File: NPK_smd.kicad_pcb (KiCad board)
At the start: 2 copper layers, 64.2 x 85.9 mm, 59 parts, among them J1 DHT, J2 Screw_Terminal_01x04, J3 USB_C_Receptacle_USB2.0_16P, Q3 SS8050, Q4 SS8050, SW1 SW_Push, SW2 SW_Push, SW3 SW_SPST, U1 AMS1117-3.3, U2 MAX485ESA_T, U3 LM2596S-ADJ, U4 ESP32-WROOM-32, U6 USBLC6-2SC6, U7 CH340C

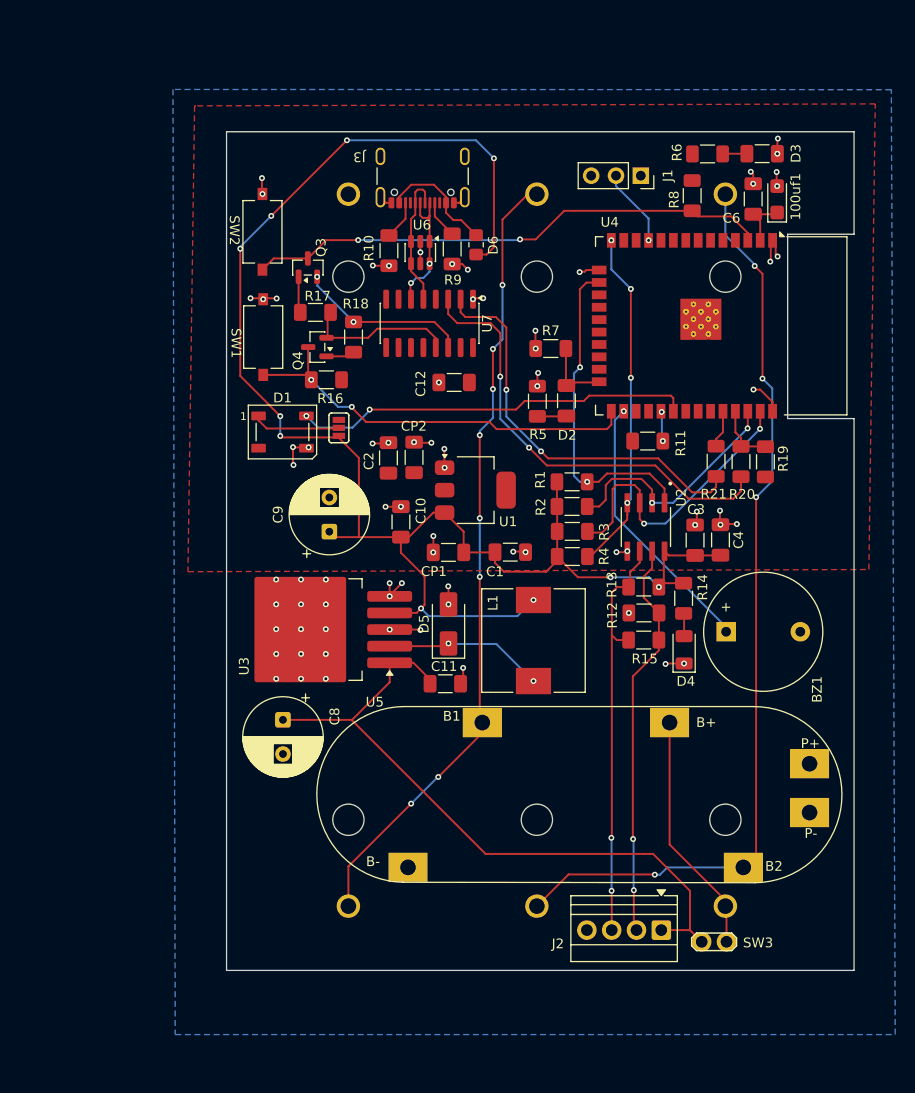
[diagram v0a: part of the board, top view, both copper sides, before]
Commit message: size minimizations and updations
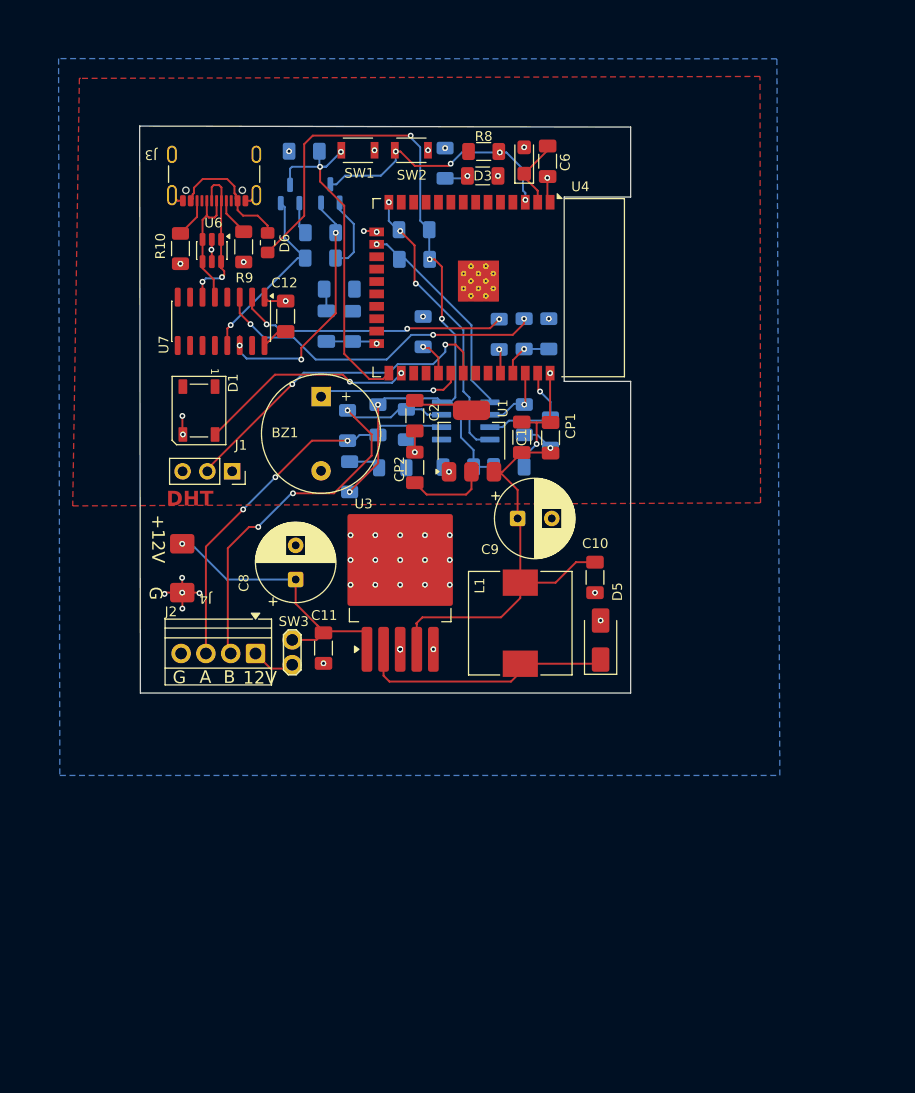
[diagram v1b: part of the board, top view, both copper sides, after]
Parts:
- removed BT2: BK-18650-PC6, 18650-3cell holder:BAT_BK-18650-PC6
- removed JP1: Jumper_3_Open, PCM_SparkFun-Jumper:Jumper_3_NO
- removed U5: ~, custom:BMS-10A-3S
- added G***: LOGO, LOGO, B.Cu at (130.1, 87.3)
- added G***: LOGO, LOGO, B.Cu at (106.3, 60.2)
- added J4: Conn_01x02_Pin, custom:solder-pad, F.Cu at (104.9, 88.3)
- added REF**: ESD-Logo_6.6x6mm_SilkScreen, Symbol:ESD-Logo_6.6x6mm_SilkScreen, B.Cu at (106.0, 69.3)
- C3, C4, D2, D4, Q3, Q4, R1, R11, R12, R13, R14, R15, R16, R17, R18, R19, R2, R20, R21, R3, R4, R5, R6, R7, U2: moved to B.Cu
- SW1, SW2: footprint Button_Switch_SMD:SW_Tactile_SPST_NO_Straight_CK_PTS636Sx25SMTRLFS -> tactile-switch:SW_B3U-1000PM
- moved J1 51.6 mm to (108.8, 75.0)
- moved SW3 50.6 mm to (115.0, 94.8), turned to 90 degrees
- moved J2 50.3 mm to (111.2, 93.7)
- moved BZ1 48.0 mm to (117.9, 67.4), turned to -90 degrees
- moved R15 37.4 mm to (120.6, 70.3), turned to 90 degrees
- moved R4 37.2 mm to (127.5, 50.3), turned to 0 degrees
- moved R14 36.4 mm to (120.8, 75.6), turned to -90 degrees
- moved D4 35.2 mm to (125.3, 74.7), turned to 180 degrees
- moved R13 32.2 mm to (123.8, 69.8), turned to 90 degrees
- moved R12 31.0 mm to (126.7, 70.2), turned to 90 degrees
- moved D3 28.7 mm to (134.5, 44.8)
- moved R1 27.9 mm to (127.5, 53.3), turned to 0 degrees
- moved R6 26.9 mm to (130.6, 43.5), turned to 90 degrees
- moved 100uf1 26.2 mm to (138.7, 43.2)
- moved R20 25.8 mm to (138.7, 60.9), turned to -90 degrees
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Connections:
- D1 pad 1: Net-(D1-VDD) -> 3V3
- U4 pad 11: /DHT -> unconnected-(U4-IO26-Pad11)
- U4 pad 26: /buz -> /WS28
- U4 pad 30: /WS28 -> /buz
- U4 pad 31: unconnected-(U4-IO19-Pad31) -> /DHT
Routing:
- net /B2: track 95.0 -> 0.00 mm, vias 4 -> 0
- net /B1: track 81.7 -> 0.00 mm, vias 8 -> 0
- net /12V: track 95.8 -> 35.1 mm, vias 0 -> 1
- net 5V: track 167.1 -> 130.0 mm, vias 10 -> 6
- net ESP32_EN: track 53.9 -> 27.0 mm, vias 2 -> 4
- net /DHT: track 8.01 -> 34.7 mm, vias 1 -> 2
- net GND: track 62.5 -> 37.2 mm, vias 75 -> 44
- net /IO23: track 30.9 -> 11.7 mm, vias 2 -> 1
- net 3V3: track 5.56 -> 24.4 mm, vias 0 -> 4
- net /WS28: track 40.9 -> 22.4 mm
- net /IO22: track 25.2 -> 7.28 mm, vias 2 -> 1
- net Net-(U7-TXD): track 41.8 -> 28.0 mm, vias 2 -> 3
- net /IO13: track 33.6 -> 22.0 mm, vias 2 -> 1
- net Net-(U7-RXD): track 46.3 -> 34.8 mm, vias 2 -> 3
- net /buz: track 27.7 -> 16.3 mm
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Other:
- board size 64.2 x 85.9 mm -> 50.3 x 58 mm
- board text added: "+12V"
- board text added: "12V"
- board text added: "A"
- board text added: "B"
- board text added: "DHT"
- board text added: "G"
